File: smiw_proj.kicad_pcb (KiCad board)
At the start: 2 copper layers, 129.5 x 93.3 mm, 48 parts, among them J1 Conn_02x06_Odd_Even, J2 Conn_02x05_Odd_Even, J3 Conn_01x02, J4 Conn_01x02, J5 Conn_02x05_Odd_Even, J6 Molex 104031, J7 Conn_02x06_Odd_Even, M1 JGB37-520, SW1 SW_Push, U1 LM2596S-5, U2 M5 Stamp-S3, U3 LD1117S33TR_SOT223, U4 L298N

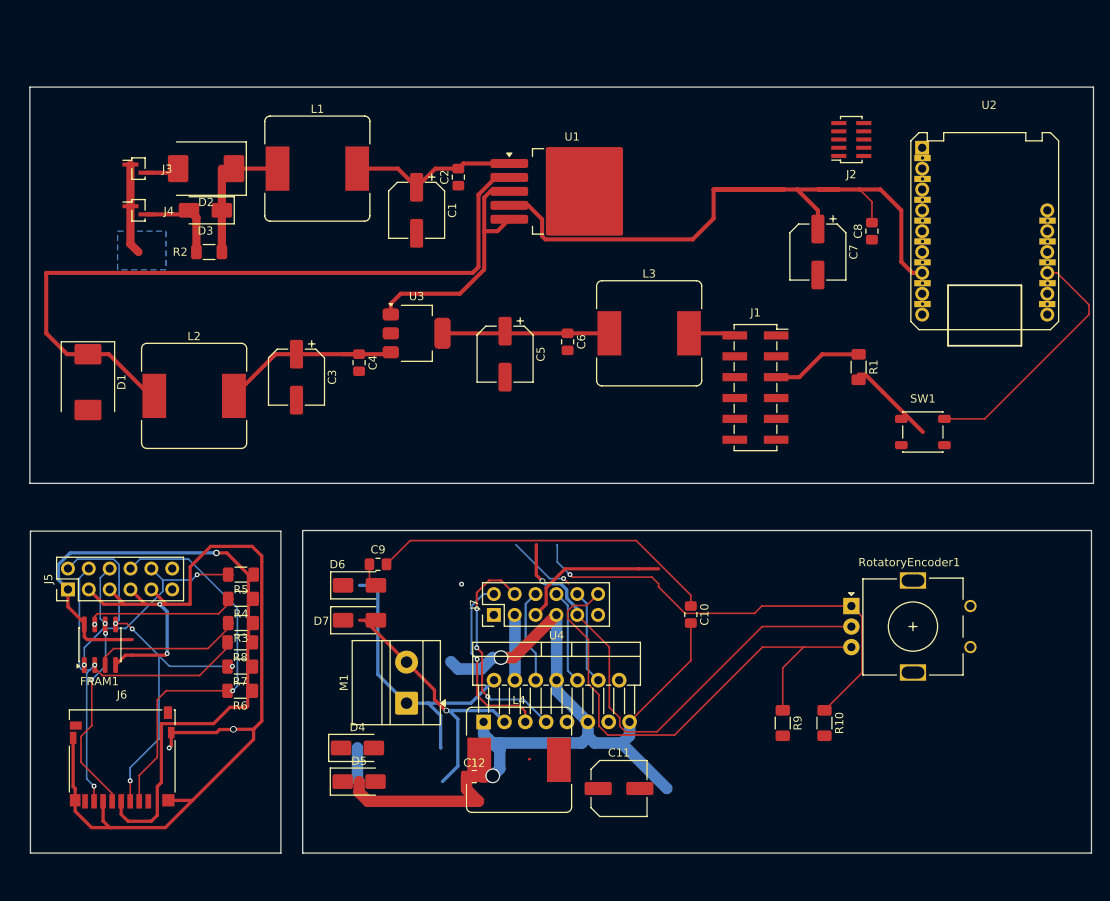
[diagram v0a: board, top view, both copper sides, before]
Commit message: już prawie, jedno sprawdzenie
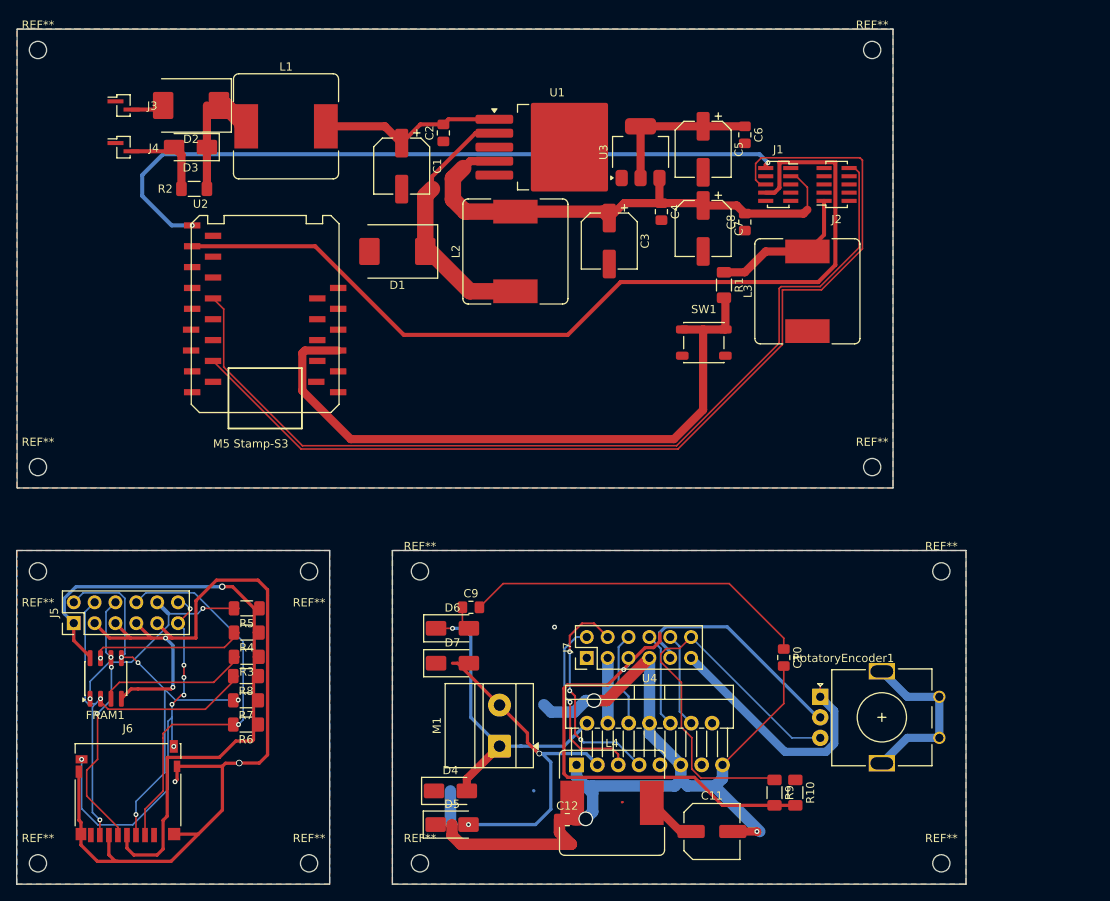
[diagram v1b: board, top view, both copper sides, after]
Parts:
- added REF**: MountingHole_2.1mm, MountingHole:MountingHole_2.1mm, F.Cu at (64.3, 78.7)
- added REF**: MountingHole_2.1mm, MountingHole:MountingHole_2.1mm, F.Cu at (17.8, 66.0)
- added REF**: MountingHole_2.1mm, MountingHole:MountingHole_2.1mm, F.Cu at (119.4, 66.0)
- added REF**: MountingHole_2.1mm, MountingHole:MountingHole_2.1mm, F.Cu at (127.8, 78.7)
- added REF**: MountingHole_2.1mm, MountingHole:MountingHole_2.1mm, F.Cu at (50.8, 114.3)
- added REF**: MountingHole_2.1mm, MountingHole:MountingHole_2.1mm, F.Cu at (17.8, 15.2)
- added REF**: MountingHole_2.1mm, MountingHole:MountingHole_2.1mm, F.Cu at (119.4, 15.2)
- added REF**: MountingHole_2.1mm, MountingHole:MountingHole_2.1mm, F.Cu at (17.8, 78.7)
- added REF**: MountingHole_2.1mm, MountingHole:MountingHole_2.1mm, F.Cu at (64.3, 114.3)
- added REF**: MountingHole_2.1mm, MountingHole:MountingHole_2.1mm, F.Cu at (50.8, 78.7)
- added REF**: MountingHole_2.1mm, MountingHole:MountingHole_2.1mm, F.Cu at (17.8, 114.3)
- added REF**: MountingHole_2.1mm, MountingHole:MountingHole_2.1mm, F.Cu at (127.8, 114.3)
- J1: footprint Connector_PinSocket_2.54mm:PinSocket_2x06_P2.54mm_Vertical_SMD -> Connector_PinSocket_1.00mm:PinSocket_2x05_P1.00mm_Vertical_SMD
- U2: footprint Library:M5Stamp-S3 -> Library2:Stamp-S3_PIN1.27_Socket
- moved U2 91.5 mm to (45.5, 47.4)
- moved L2 42.9 mm to (75.9, 39.8), turned to 90 degrees
- moved C3 41.5 mm to (87.4, 38.5)
- moved C4 41.2 mm to (93.7, 34.9)
- moved D1 40.9 mm to (61.6, 39.8), turned to 180 degrees
- moved U3 35.1 mm to (91.2, 27.7), turned to 90 degrees
- moved C5 34.7 mm to (98.8, 27.3)
- moved C6 33.2 mm to (103.9, 25.6)
- moved SW1 28.8 mm to (98.9, 50.9)
- moved J1 24.9 mm to (107.9, 31.6)
- moved L3 19.9 mm to (111.5, 44.6), turned to 90 degrees
- moved R1 19.2 mm to (101.3, 43.9)
- moved C8 15.5 mm to (103.9, 36.2)
- moved C7 14.3 mm to (98.8, 37.0)
- moved C11 12.5 mm to (99.9, 110.4)
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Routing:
- net /PWM A: track 11.5 -> 136.7 mm
- net /~{FRAM CS}: track 0.00 -> 114.7 mm
- net /DRIVER IN3: track 11.6 -> 122.2 mm
- net /DRIVER IN1: track 22.5 -> 111.0 mm, vias 1 -> 3
- net (no net): track 0.00 -> 70.0 mm, vias 0 -> 7
- net Net-(D1-K): track 90.1 -> 31.3 mm
- net Vcc: track 118.6 -> 70.5 mm
- net GND: track 255.2 -> 214.7 mm, vias 6 -> 7
- net Vdd: track 35.2 -> 75.1 mm, vias 0 -> 1
- net /reset: track 41.5 -> 80.8 mm
- net CPU_GND: track 61.2 -> 28.0 mm, vias 1 -> 0
- net /ENC A: track 56.3 -> 30.2 mm, vias 1 -> 0
- net /ENC B: track 72.9 -> 50.6 mm, vias 1 -> 0
- net Net-(D5-A): track 33.7 -> 41.8 mm, vias 1 -> 2
- net VDD: track 128.6 -> 121.1 mm
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- added copper zone on F.Cu, net GND
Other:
- board size 129.5 x 93.3 mm -> 115.6 x 104.1 mm
